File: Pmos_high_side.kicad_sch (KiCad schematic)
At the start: 31 parts, among them Q1 PMOS, Q10 AO3401A, Q11 MMBT5401 200-300, Q12 MMBT5551 200-300, Q14 MMBT5551 200-300, Q9 MMBT5551 200-300

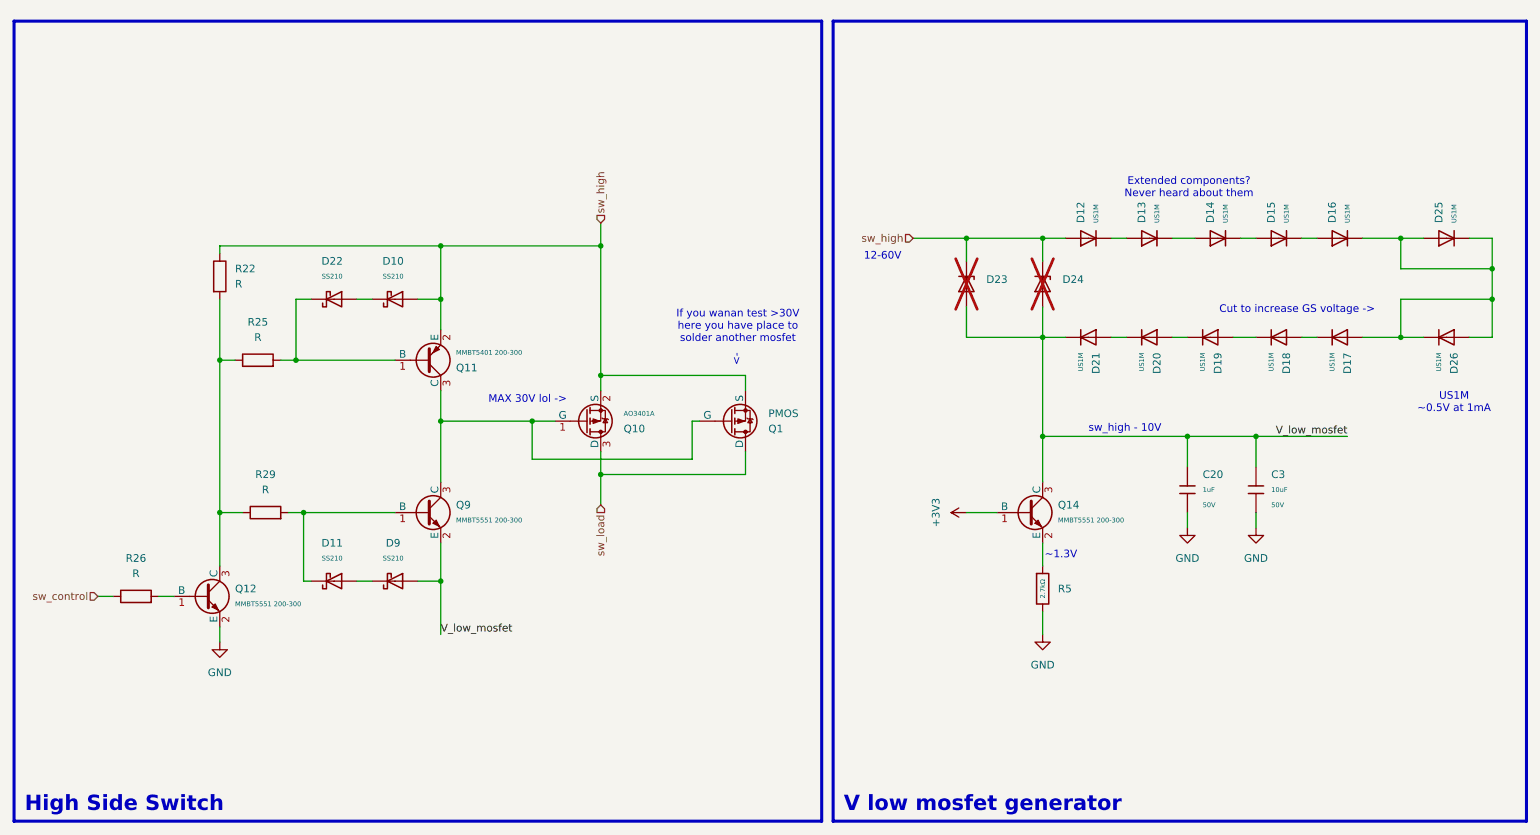
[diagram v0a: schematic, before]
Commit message: finished routing
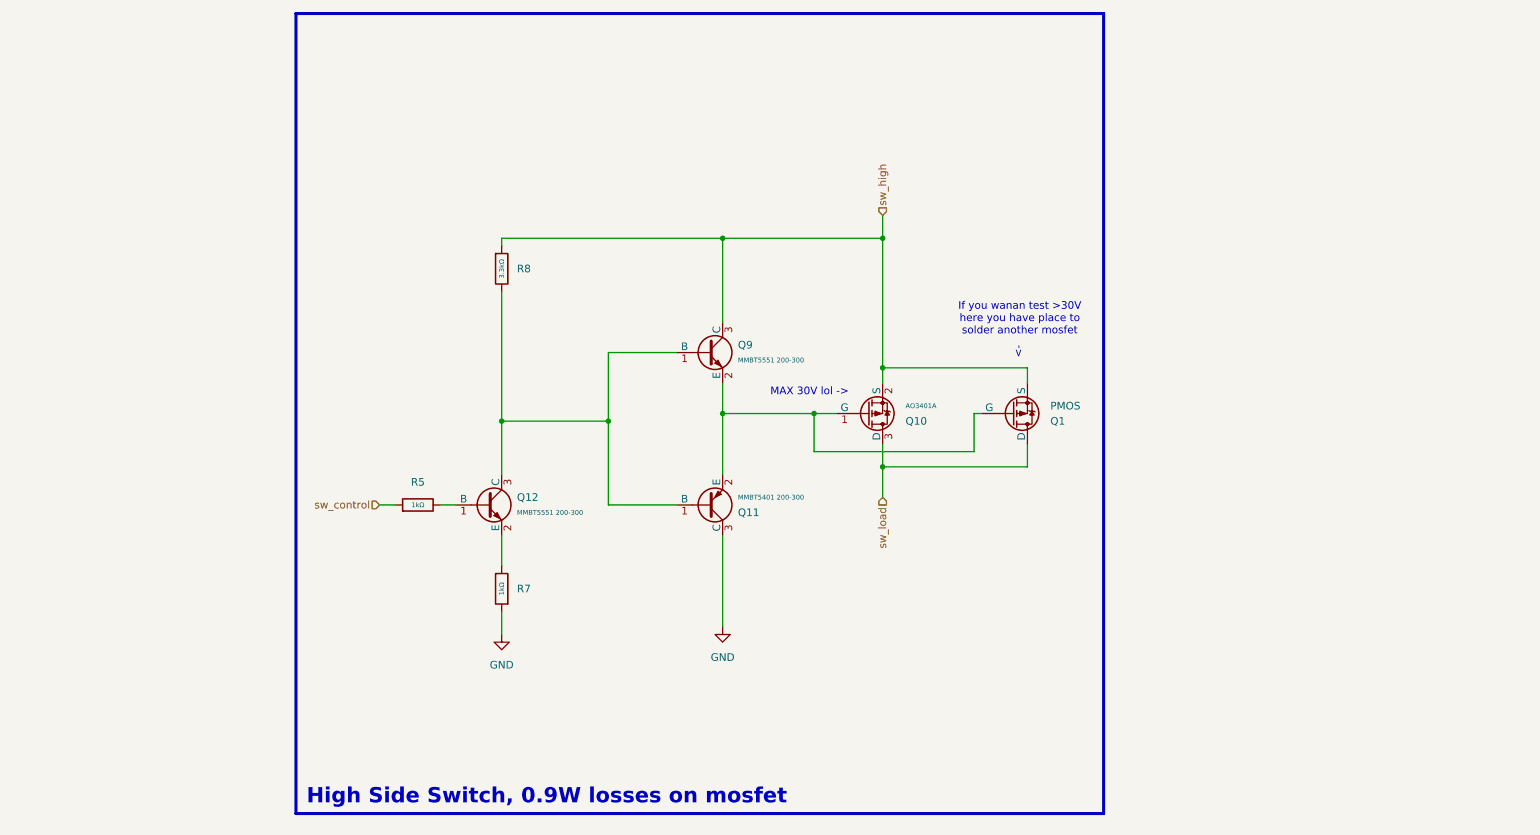
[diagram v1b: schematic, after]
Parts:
- removed C20: 1uF, PCM_JLCPCB:C_0603, symbol PCM_JLCPCB-Capacitors:0603,1uF
- removed C3: 10uF, PCM_JLCPCB:C_1206, symbol PCM_JLCPCB-Capacitors:1206,10uF
- removed D10, D11, D22, D9: SS210, PCM_JLCPCB:D_SMA, symbol PCM_JLCPCB-Diodes:Schottky,SS210
- removed D12, D13, D14, D15, D16, D17, D18, D19, D20, D21, D25, D26: US1M, PCM_JLCPCB:D_SMA, symbol PCM_JLCPCB-Diodes:Recovery,US1M
- removed D23: D_Zener, Diode_SMD:D_SOD-123, symbol Device:D_Zener
- removed D24: D_Zener, Diode_THT:D_DO-15_P2.54mm_Vertical_AnodeUp, symbol Device:D_Zener
- removed Q14: MMBT5551 200-300, PCM_JLCPCB:Q_SOT-23, symbol PCM_JLCPCB-Transistors:NPN,MMBT5551 200-300
- removed R22, R25, R26, R29: R, symbol Device:R
- removed R5: 2.7kΩ, PCM_JLCPCB:R_0603, symbol PCM_JLCPCB-Resistors:0603,2.7kΩ
- added R5, R7: 1kΩ, PCM_JLCPCB:R_0603, symbol PCM_JLCPCB-Resistors:0603,1kΩ
- added R8: 3.3kΩ, PCM_JLCPCB:R_0603, symbol PCM_JLCPCB-Resistors:0603,3.3kΩ
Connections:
- net V_low_mosfet is gone; now on an unnamed net: Q9.2 (E)
- net GND: now also Q11.3 (C), R7.1; no longer Q12.2 (E)
- net sw_control: now also R5.1
- net sw_high: now also Q9.3 (C), R8.1; no longer Q11.2 (E)
- net at Q12.1 (B): now also R5.2
- net at Q1.2 (G), Q10.1 (G): now also Q11.2 (E); no longer Q11.3 (C), Q9.3 (C)
- net at Q12.3 (C): now also Q11.1 (B), Q9.1 (B), R8.2
- new net: Q12.2 (E), R7.2
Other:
- note added: "High Side Switch, 0.9W losses on mosfet"
- note removed: "12-60V"
- note removed: "Cut to increase GS voltage ->"
- note removed: "Extended components? Never heard about them"
- note removed: "High Side Switch"
- note removed: "US1M ~0.5V at 1mA"
- note removed: "V low mosfet generator"
- note removed: "sw_high - 10V"
- note removed: "~1.3V"
- moved on the sheet: Q1, Q10, Q12
